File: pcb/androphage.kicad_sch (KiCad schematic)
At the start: 62 parts

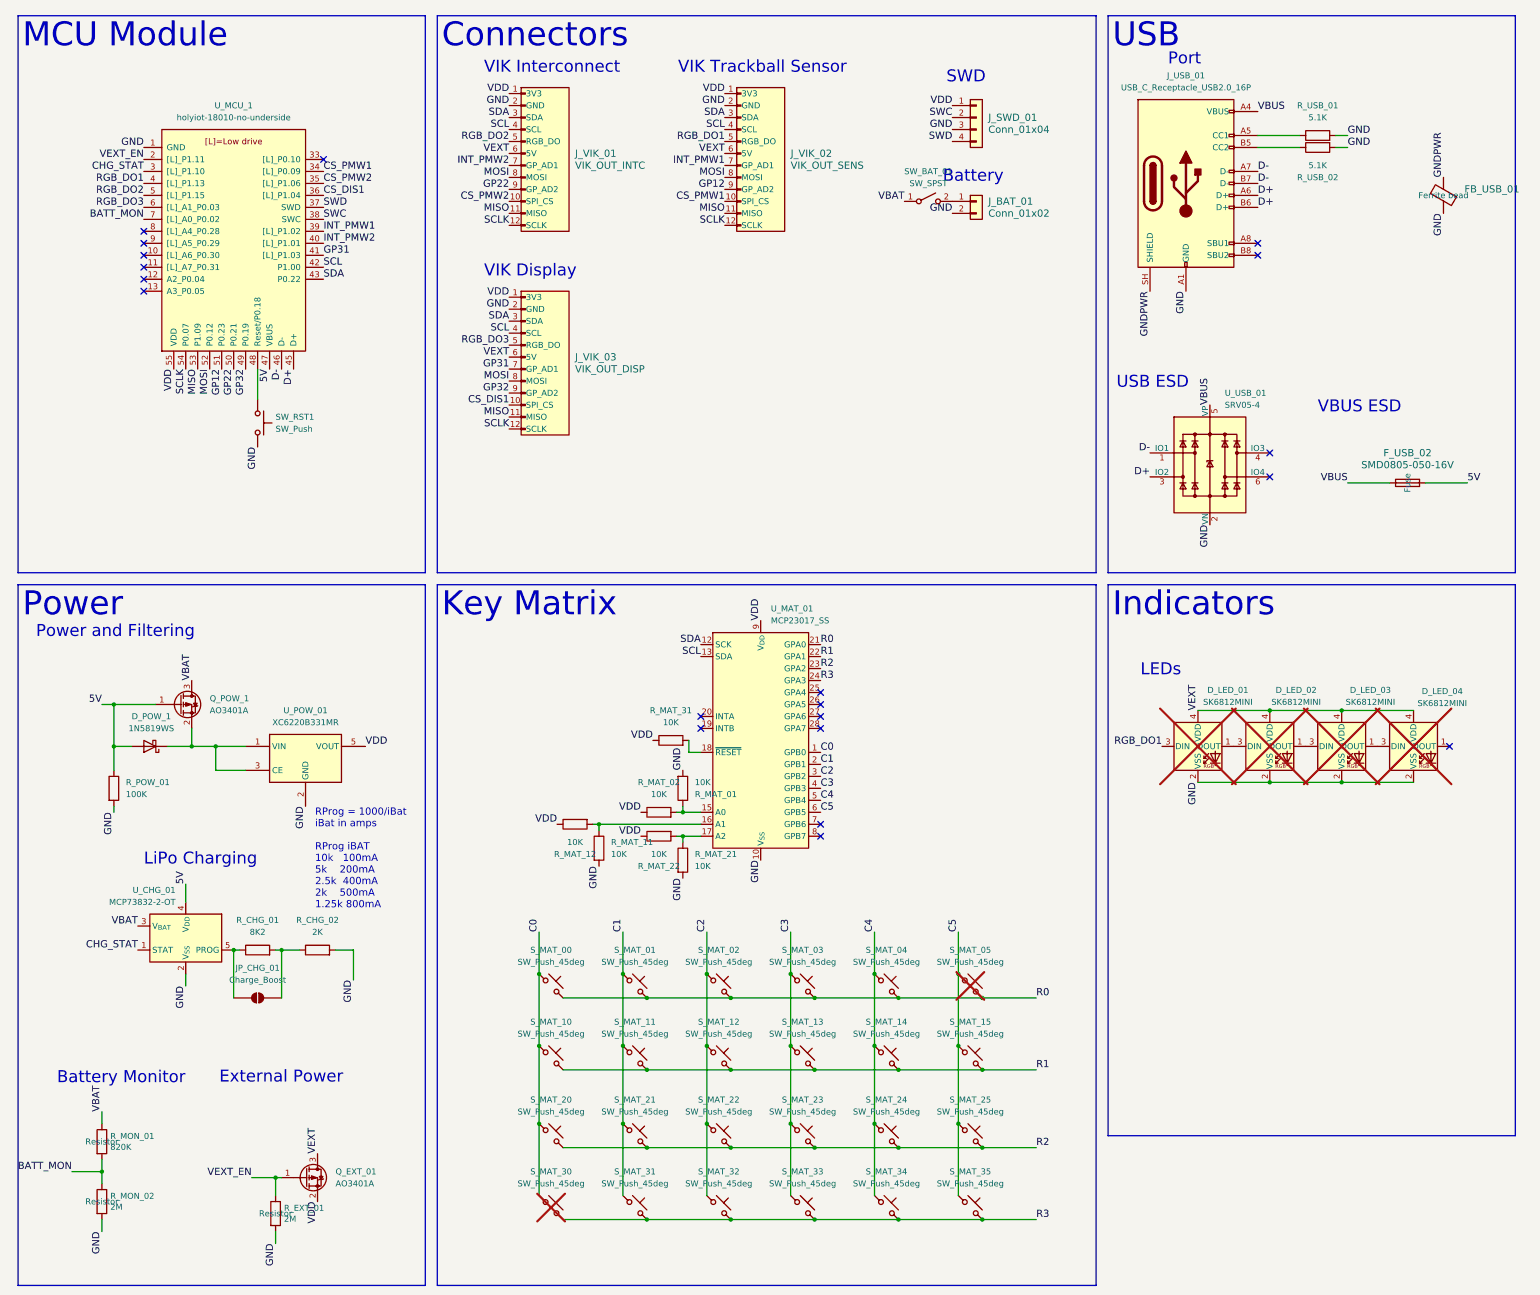
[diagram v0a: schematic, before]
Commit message: Work on PCBs.
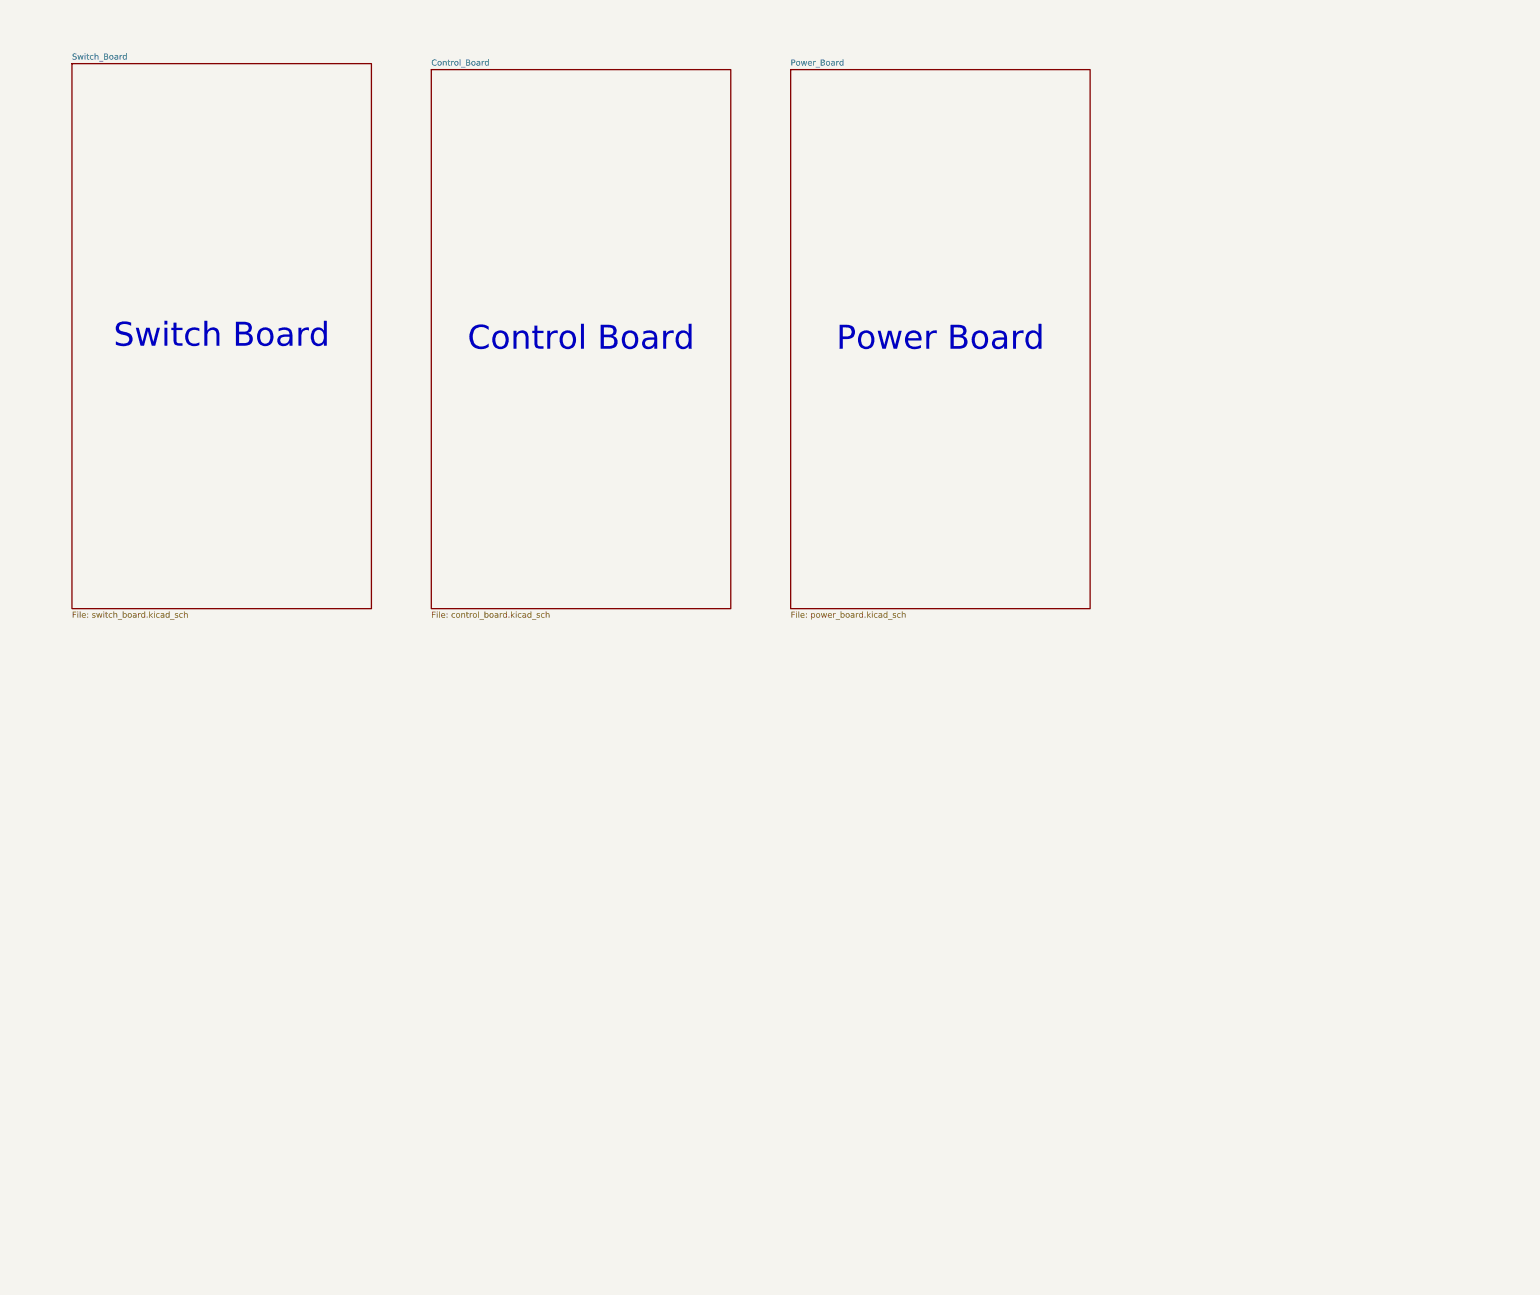
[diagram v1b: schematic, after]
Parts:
- removed D_LED_01, D_LED_02, D_LED_03, D_LED_04: SK6812MINI, LED_SMD:LED_SK6812MINI_PLCC4_3.5x3.5mm_P1.75mm, symbol LED:SK6812MINI
- removed D_POW_1: 1N5819WS, Diode_SMD:D_SOD-323, symbol Diode:1N5819WS
- removed FB_USB_01: (no value), Inductor_SMD:L_0805_2012Metric, symbol Device:FerriteBead
- removed F_USB_02: SMD0805-050-16V, Fuse:Fuse_0805_2012Metric, symbol Device:Fuse
- removed JP_CHG_01: Charge_Boost, Jumper:SolderJumper-2_P1.3mm_Open_RoundedPad1.0x1.5mm, symbol Jumper:SolderJumper_2_Open
- removed J_BAT_01: Conn_01x02, Connector_JST:JST_GH_SM02B-GHS-TB_1x02-1MP_P1.25mm_Horizontal, symbol Connector_Generic:Conn_01x02
- removed J_SWD_01: Conn_01x04, Connector_PinSocket_2.54mm:PinSocket_1x04_P2.54mm_Vertical, symbol Connector_Generic:Conn_01x04
- removed J_USB_01: USB_C_Receptacle_USB2.0_16P, Connector_USB:USB_C_Receptacle_HRO_TYPE-C-31-M-12, symbol Connector:USB_C_Receptacle_USB2.0_16P
- removed J_VIK_01: VIK_OUT_INTC, vik:vik-keyboard-connector-horizontal, symbol vik:vik-keyboard-connector
- removed J_VIK_02: VIK_OUT_SENS, vik:vik-keyboard-connector-horizontal, symbol vik:vik-keyboard-connector
- removed J_VIK_03: VIK_OUT_DISP, vik:vik-keyboard-connector-horizontal, symbol vik:vik-keyboard-connector
- removed Q_EXT_01, Q_POW_1: AO3401A, Package_TO_SOT_SMD:SOT-23, symbol Transistor_FET:AO3401A
- removed R_CHG_01: 8K2, Resistor_SMD:R_0201_0603Metric_Pad0.64x0.40mm_HandSolder, symbol Device:R
- removed R_CHG_02: 2K, Resistor_SMD:R_0201_0603Metric_Pad0.64x0.40mm_HandSolder, symbol Device:R
- removed R_EXT_01, R_MON_02: 2M, Resistor_SMD:R_0603_1608Metric, symbol Device:R
- removed R_MAT_01, R_MAT_02, R_MAT_11, R_MAT_12, R_MAT_21, R_MAT_22, R_MAT_31: 10K, Resistor_SMD:R_0201_0603Metric_Pad0.64x0.40mm_HandSolder, symbol Device:R
- removed R_MON_01: 820K, Resistor_SMD:R_0603_1608Metric, symbol Device:R
- removed R_POW_01: 100K, Resistor_SMD:R_0201_0603Metric_Pad0.64x0.40mm_HandSolder, symbol Device:R
- removed R_USB_01, R_USB_02: 5.1K, Resistor_SMD:R_0201_0603Metric_Pad0.64x0.40mm_HandSolder, symbol Device:R
- removed SW_BAT_01: SW_SPST, library:AS11CH, symbol Switch:SW_SPST
- removed SW_RST1: SW_Push, Button_Switch_SMD:SW_Push_1P1T_NO_E-Switch_TL3301NxxxxxG, symbol Switch:SW_Push
- removed S_MAT_00, S_MAT_01, S_MAT_02, S_MAT_03, S_MAT_04, S_MAT_10, S_MAT_11, S_MAT_12, S_MAT_13, S_MAT_14, S_MAT_15, S_MAT_20, S_MAT_21, S_MAT_22, S_MAT_23, S_MAT_24, S_MAT_25, S_MAT_31, S_MAT_32, S_MAT_33, S_MAT_34, S_MAT_35: SW_Push_45deg, key-switches:SW_Kailh_Choc_V1V2_HotSwap_PTH_Double, symbol Switch:SW_Push_45deg
- removed S_MAT_05, S_MAT_30: SW_Push_45deg, symbol Switch:SW_Push_45deg
- removed U_CHG_01: MCP73832-2-OT, Package_TO_SOT_SMD:SOT-23-5, symbol Battery_Management:MCP73832-2-OT
- removed U_MAT_01: MCP23017_SS, Package_SO:SSOP-28_5.3x10.2mm_P0.65mm, symbol Interface_Expansion:MCP23017x-x-SS
- removed U_MCU_1: holyiot-18010-no-underside, mcu:holyiot-18010-no-underside, symbol mcu:holyiot-18010-no-underside
- removed U_POW_01: XC6220B331MR, Package_TO_SOT_SMD:SOT-23-5, symbol Regulator_Linear:XC6220B331MR
- removed U_USB_01: SRV05-4, Package_TO_SOT_SMD:SOT-23-6, symbol Power_Protection:SRV05-4
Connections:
- no-connect marks 20 -> 0
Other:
- added sheet Control_Board (control_board.kicad_sch)
- added sheet Power_Board (power_board.kicad_sch)
- added sheet Switch_Board (switch_board.kicad_sch)
- note added: "Control Board"
- note added: "Power Board"
- note added: "Switch Board"
- note removed: "Battery"
- note removed: "Battery Monitor"
- note removed: "External Power"
- note removed: "LEDs"
- note removed: "LiPo Charging"
- note removed: "Port"
- note removed: "Power and Filtering"
- note removed: "RProg = 1000/iBat iBat in amps RProg iBAT 10k 100mA 5k 200mA 2.5k 400mA 2k 500mA 1.25k 800mA"
- note removed: "SWD"
- note removed: "USB ESD"
- note removed: "VBUS ESD"
- note removed: "VIK Display"
- note removed: "VIK Interconnect"
- note removed: "VIK Trackball Sensor"
